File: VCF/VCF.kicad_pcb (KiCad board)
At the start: 2 copper layers, 99.3 x 128 mm, 56 parts, among them J1 Conn_01x10_Pin, J2 Conn_01x10_Pin, J3 Conn_01x06_Pin, Q1 BC557, Q2 BC557, Q3 BC547, U1 Aux_flush, U10 Aux_flush, U11 Aux_flush, U2 Aux_flush, U3 TL074, U4 TL072, U5 LM13700, U6 Aux_flush, U7 Aux_flush, U9 Aux_flush

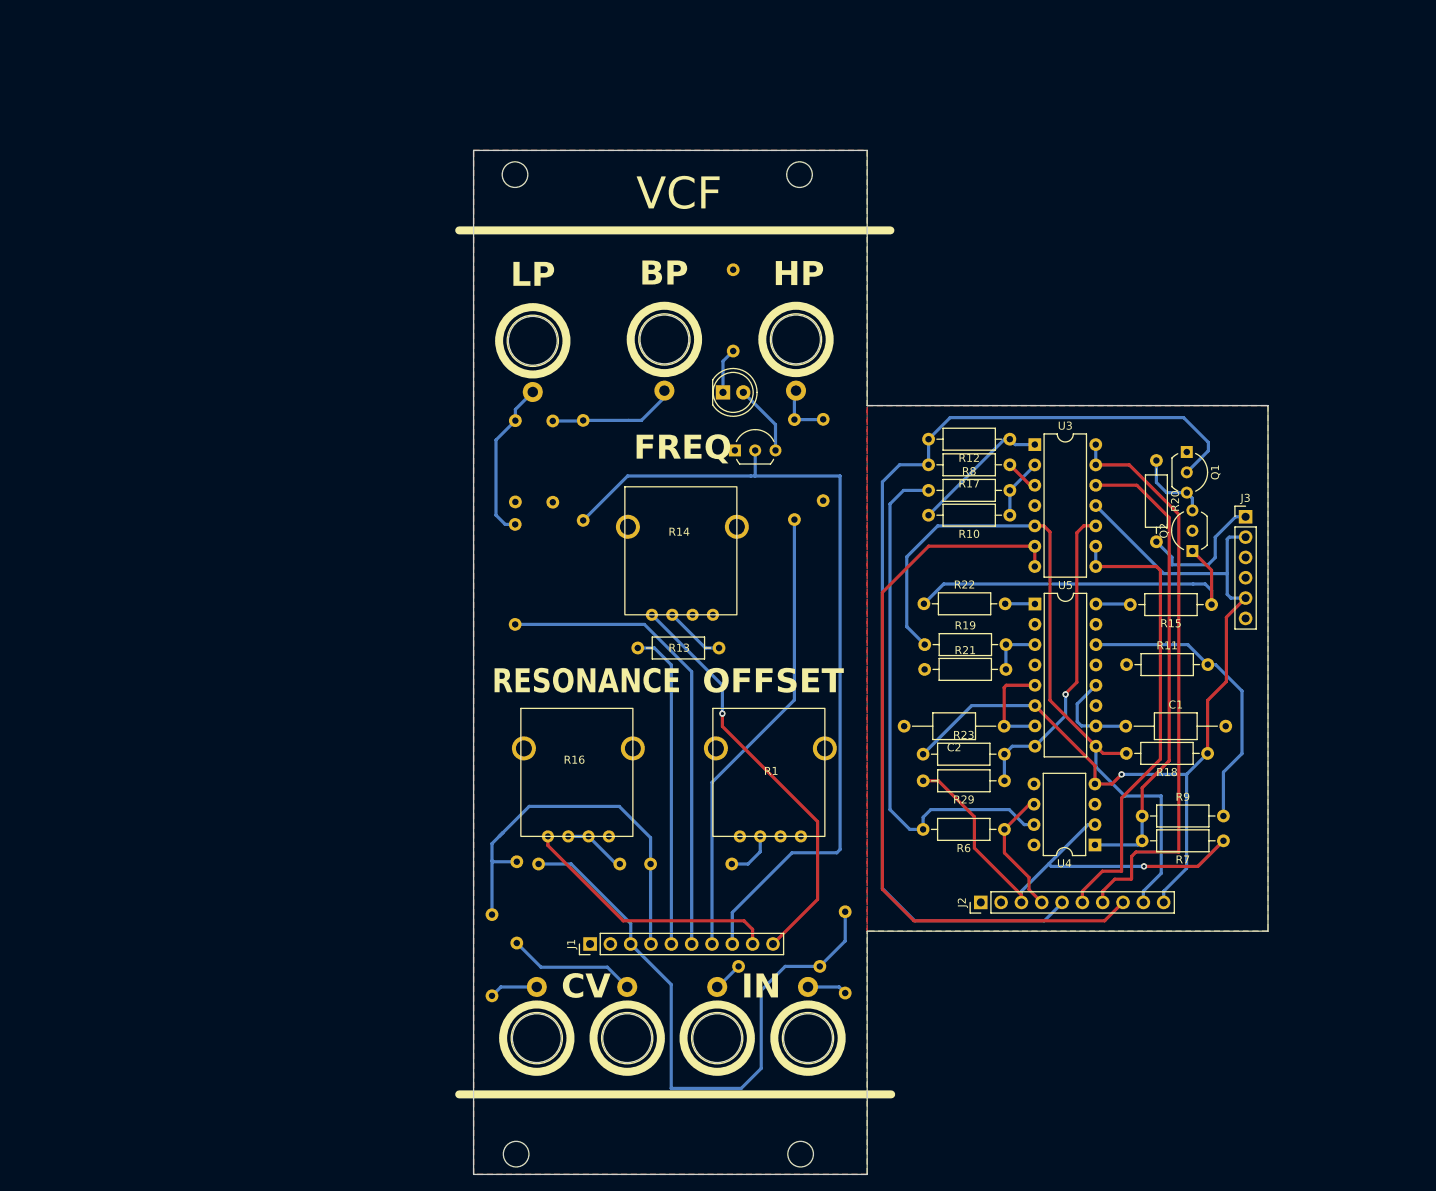
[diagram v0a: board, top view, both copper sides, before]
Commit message: Add files via upload
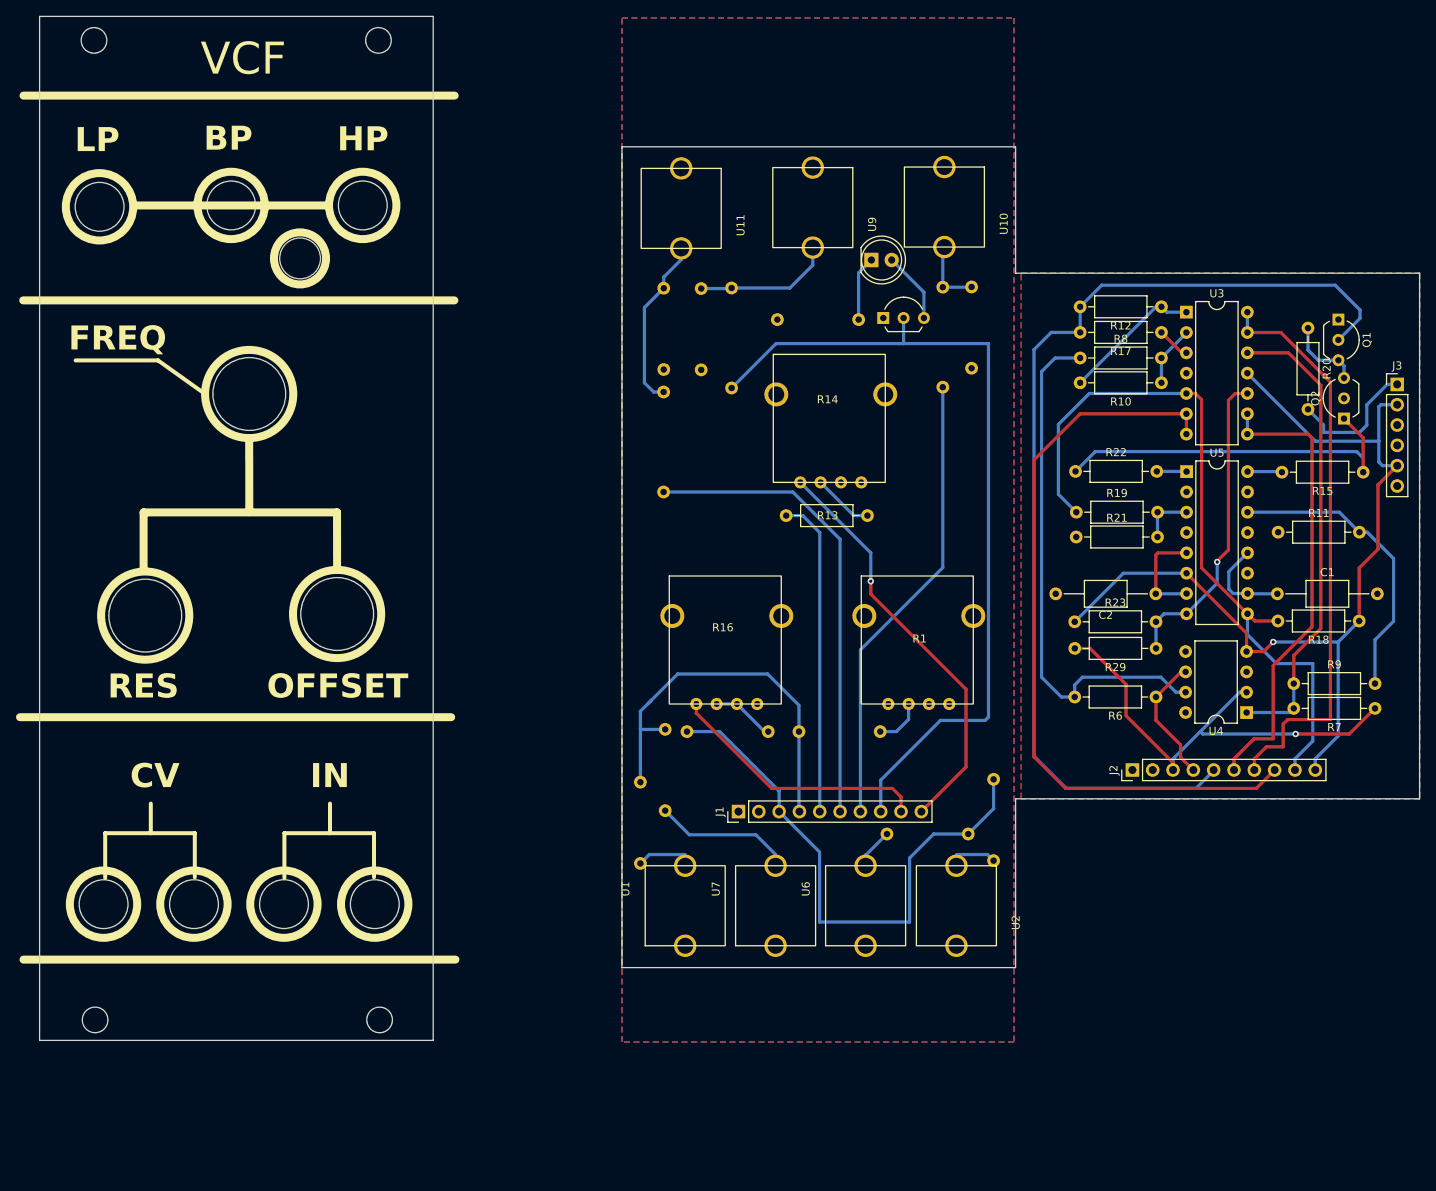
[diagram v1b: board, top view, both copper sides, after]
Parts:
- added ?: , , F.Cu at (98.1, 134.2)
- added ?: , , F.Cu at (93.8, 70.5)
- added ?: , , F.Cu at (100.1, 53.5)
- added ?: , , F.Cu at (108.0, 46.9)
- added ?: , , F.Cu at (86.8, 134.2)
- added ?: , , F.Cu at (104.7, 98.0)
- added ?: , , F.Cu at (80.8, 98.2)
- added ?: , , F.Cu at (91.5, 46.9)
- added ?: , , F.Cu at (109.5, 134.2)
- added ?: , , F.Cu at (75.0, 47.0)
- added ?: , , F.Cu at (75.5, 134.2)
- R21: value 100k -> 1k
- U1, U10, U11, U2, U6, U7, U9: footprint Library:aux_flush -> Library:3mm5 Mono Aux
- moved REF** 55.2 mm to (74.5, 148.7)
- moved REF** 55.2 mm to (74.3, 26.2)
- moved REF** 55.2 mm to (109.9, 26.2)
- moved REF** 55.2 mm to (110.0, 148.7)
- moved Q1 25.2 mm to (229.9, 61.1)
- moved R11 25.2 mm to (222.4, 87.7)
- moved U3 25.2 mm to (210.9, 60.2)
- moved C1 25.2 mm to (222.3, 95.4)
- moved J2 25.2 mm to (204.2, 117.5)
- moved R29 25.2 mm to (207.1, 102.2)
- moved R8 25.2 mm to (197.6, 66.0)
- moved R15 25.2 mm to (233.0, 80.2)
- moved R19 25.2 mm to (197.1, 85.2)
- moved R20 25.2 mm to (226.1, 62.2)
- moved C2 25.2 mm to (207.1, 95.4)
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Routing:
- net VGND2: track 134.8 -> 127.7 mm
- net Net-(D1-K): track 5.70 -> 8.11 mm
- net Net-(C4-Pad2): track 7.60 -> 9.00 mm
- net Net-(C5-Pad2): track 20.3 -> 21.7 mm
- net Net-(C3-Pad2): track 16.3 -> 17.3 mm
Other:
- board size 99.3 x 128 mm -> 172.5 x 128 mm
- board text added: "RES"
- board text removed: "RESONANCE"
